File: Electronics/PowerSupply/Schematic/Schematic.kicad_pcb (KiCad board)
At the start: 2 copper layers, 145 x 110 mm, 95 parts, among them J1 +12V, J2 GND, J3 Scope, J4 Disable, J5 XDUCER, K1 RELAY, P1 I1, P10 CONN_1, P11 CONN_1, P12 CONN_1, P13 CONN_1, P14 CONN_1, P15 CONN_1, P16 CONN_1, P17 CONN_1, P18 CONN_1, P19 CONN_1, P2 I2, P20 CONN_1, P21 CONN_1, P22 CONN_1, P23 CONN_1, P24 CONN_1, P25 CONN_1, P26 CONN_1, P27 CONN_1, P28 CONN_1, P29 CONN_1, P3 LED1, P30 CONN_1, P31 TUNE, P4 LED2, P5 O2, P6 O1, P7 SMPS-UT, P8 SMPS-CT, P9 SMPS-LT, Q1 IRFB3306, Q2 IRFB3306, Q3 2N2222, T1 SMPS, U1 ACS712, U2 AD9833_Board, U3 50K, U4 10K, U5 SG3525, U6 Arduino_Nano, U7 74HC1G86, U8 OPA350

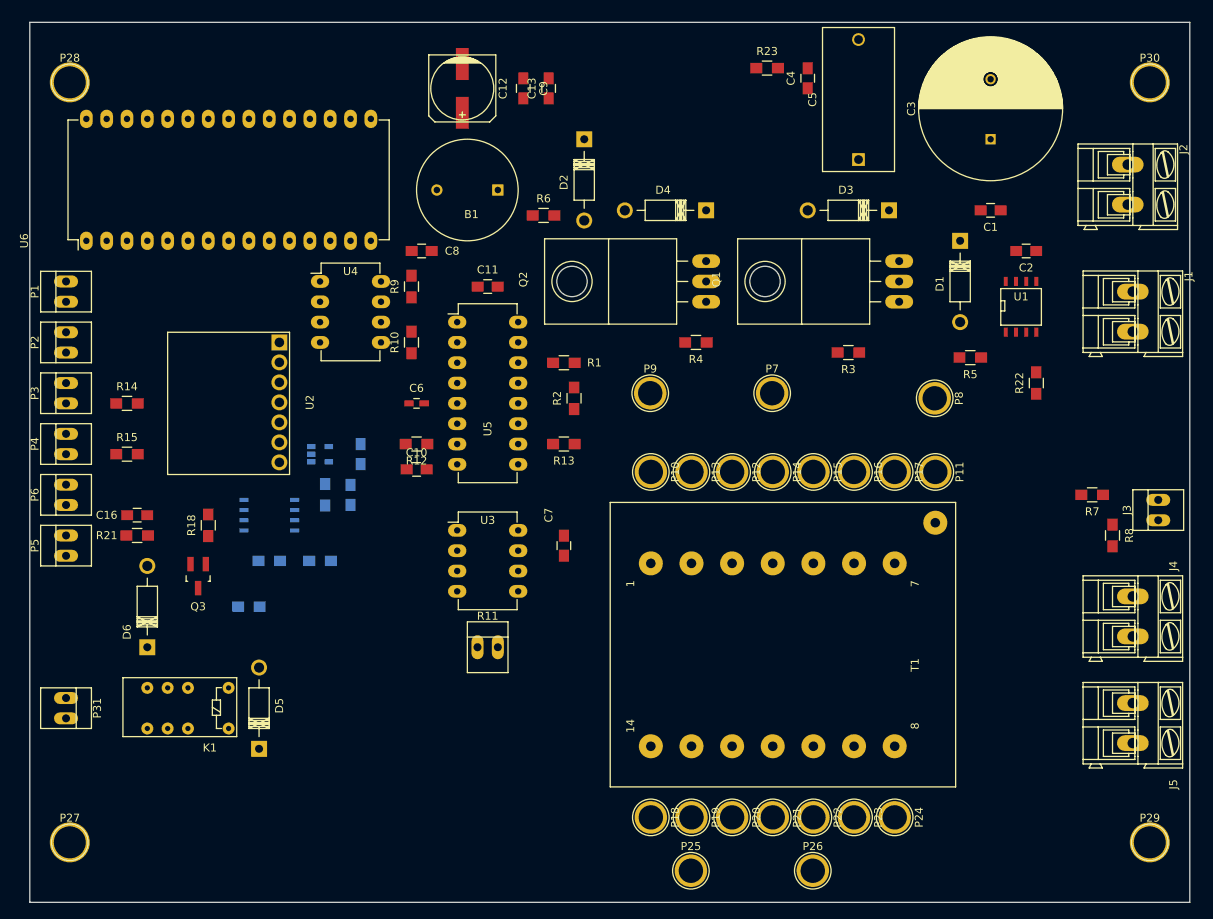
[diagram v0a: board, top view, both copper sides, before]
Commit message: Completed Board layout and generated gerber files.
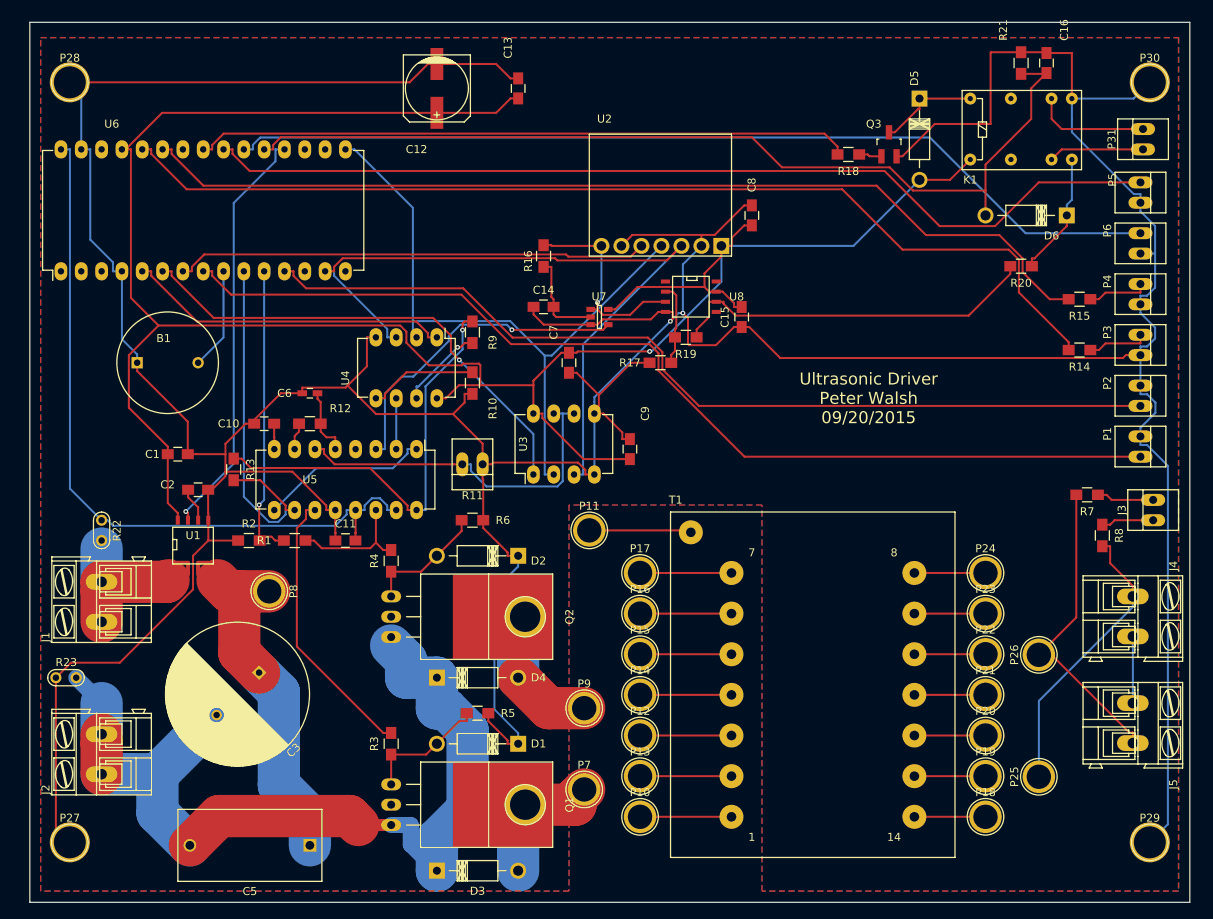
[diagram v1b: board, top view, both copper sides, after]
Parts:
- removed C4: 100nF, Capacitors_SMD:C_0805_HandSoldering
- C14, C15, R16, R17, R19, R20, U7, U8: moved to F.Cu
- Q1, Q2: footprint Transistors_TO-220:TO-220_Neutral123_Horizontal_LargePads -> TO-220:TO-220_Neutral123_Horizontal_with_tab_pad
- R22, R23: footprint Resistors_SMD:R_0805_HandSoldering -> Discret:TEST_POINT_2PADS
- moved P31 152.3 mm to (184.2, 54.6), turned to 90 degrees
- moved J2 149.2 mm to (54.0, 134.0), turned to 90 degrees
- moved P5 141.4 mm to (183.8, 61.3), turned to 270 degrees
- moved P6 137.9 mm to (183.8, 67.6), turned to 270 degrees
- moved P1 135.7 mm to (183.8, 93.0), turned to 270 degrees
- moved P4 135.6 mm to (183.8, 74.0), turned to 270 degrees
- moved J1 135.4 mm to (54.0, 114.9), turned to 90 degrees
- moved P2 134.5 mm to (183.8, 86.7), turned to 270 degrees
- moved P3 134.4 mm to (183.8, 80.3), turned to 270 degrees
- moved D6 127.0 mm to (174.6, 64.1), turned to 180 degrees
- moved C16 126.9 mm to (172.1, 45.1), turned to 90 degrees
- moved R21 125.3 mm to (168.9, 45.1), turned to 270 degrees
- moved R15 120.6 mm to (176.2, 74.6), turned to 180 degrees
- moved K1 120.0 mm to (162.6, 52.1), turned to 0 degrees
- moved R14 119.2 mm to (176.2, 81.0), turned to 180 degrees
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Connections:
- Q1 pad 2: Net-(D3-Pad2) -> (no net)
- Q2 pad 2: Net-(D4-Pad2) -> (no net)
- U1 pad 1: Net-(C3-Pad1) -> PWR-12V
- U1 pad 2: Net-(C3-Pad1) -> PWR-12V
- U1 pad 3: PWR-12V -> Net-(C3-Pad1)
- U1 pad 4: PWR-12V -> Net-(C3-Pad1)
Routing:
- net GND: track 0.00 -> 634.7 mm, vias 0 -> 2
- net +5V: track 0.00 -> 281.4 mm, vias 0 -> 1
- net Net-(R14-Pad2): track 0.00 -> 129.5 mm
- net Net-(P1-Pad2): track 0.00 -> 128.4 mm
- net Net-(R15-Pad2): track 0.00 -> 122.4 mm
- net Net-(P5-Pad1): track 0.00 -> 121.2 mm
- net UC-TUNE: track 0.00 -> 118.1 mm
- net Net-(P6-Pad1): track 0.00 -> 118.0 mm
- net PWR-GND: track 0.00 -> 115.7 mm
- net Net-(P2-Pad2): track 0.00 -> 115.6 mm
- net UC-SDA: track 0.00 -> 94.5 mm
- net +12V: track 0.00 -> 93.1 mm
- net UC-SCK: track 0.00 -> 82.6 mm
- net UC-RELAY: track 0.00 -> 82.1 mm
- net UC-CSF: track 0.00 -> 61.3 mm, vias 0 -> 1
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- added copper zone on B.Cu, net GND
- added copper zone on F.Cu, net GND
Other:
- net class HighCurrent: trace_width 4 -> 5.29
- board text added: "Ultrasonic Driver Peter Walsh 09/20/2015"
